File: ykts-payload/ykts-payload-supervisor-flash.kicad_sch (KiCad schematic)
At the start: 10 parts, among them U10 AMS1117-3.3, U11 AT25DF161-SF-T

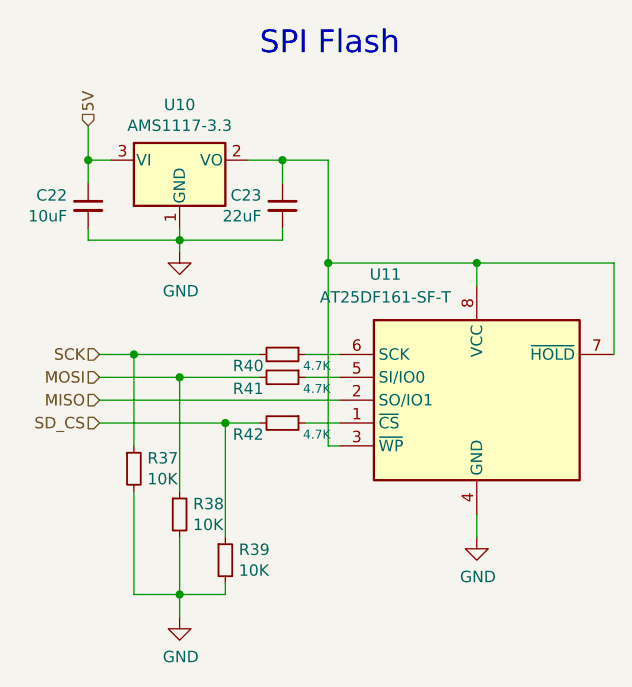
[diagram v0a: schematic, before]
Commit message: Changed flash LDO to L78L33
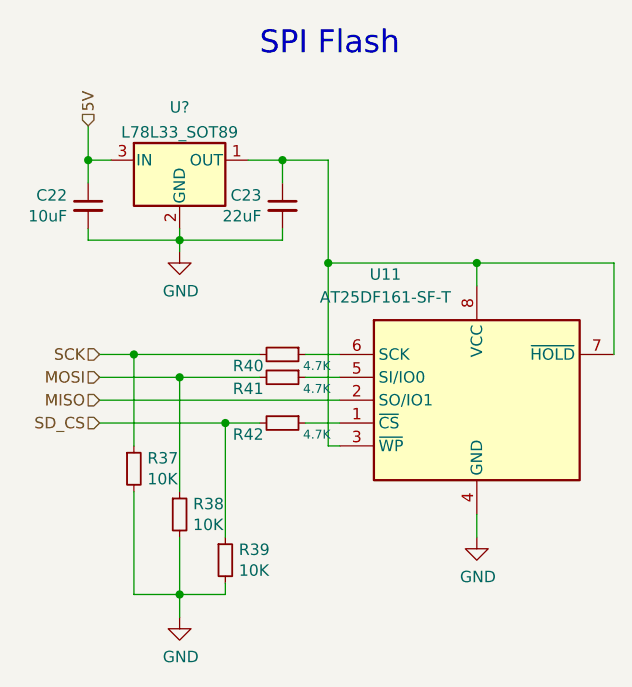
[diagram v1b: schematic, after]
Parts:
- removed U10: AMS1117-3.3, Package_TO_SOT_SMD:SOT-89-3, symbol Regulator_Linear:AMS1117-3.3
- added U?: L78L33_SOT89, Package_TO_SOT_SMD:SOT-89-3, symbol Regulator_Linear:L78L33_SOT89
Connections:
- net 5V: now also U?.3 (IN)
- net GND: now also U?.2 (GND)
- net at C23.1, U11.3 (~{WP}), U11.7 (~{HOLD})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: now also U?.1 (OUT)
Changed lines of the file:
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@@
     (pin "2")
-  )
-  (symbol (lib_id "Regulator_Linear:AMS1117-3.3") (at 132.08 74.93 0)
-    (in_bom yes) (on_board yes)
-    (property "Reference" "U10" (id 0) (at 132.08 68.7832 0))
-    (property "Value" "AMS1117-3.3" (id 1) (at 132.08 71.0946 0))
-    (property "Footprint" "Package_TO_SOT_SMD:SOT-89-3" (id 2) (at 132.08 69.85 0)
-      (effects (font (size 1.27 1.27)) hide)
-    )
-    (property "Datasheet" "http://www.advanced-monolithic.com/pdf/ds1117.pdf" (id 3) (at 134.62 81.28 0)
-      (effects (font (size 1.27 1.27)) hide)
-    )
-    (pin "1")
-    (pin "2")
-    (pin "3")
   )
   (symbol (lib_id "Device:R_Small") (at 127 109.22 0)
@@
     (pin "2")
   )
+  (symbol (lib_id "Regulator_Linear:L78L33_SOT89") (at 132.08 74.93 0)
+    (in_bom yes) (on_board yes) (fields_autoplaced)
+    (property "Reference" "U?" (id 0) (at 132.08 69.0585 0))
+    (property "Value" "L78L33_SOT89" (id 1) (at 132.08 71.8336 0))
+    (property "Footprint" "Package_TO_SOT_SMD:SOT-89-3" (id 2) (at 132.08 69.85 0)
+      (effects (font (size 1.27 1.27) italic) hide)
+    )
+    (property "Datasheet" "http://www.st.com/content/ccc/resource/technical/document/datasheet/15/55/e5/aa/23/5b/43/fd/CD00000446.pdf/files/CD00000446.pdf/jcr:content/translations/en.CD00000446.pdf" (id 3) (at 132.08 76.2 0)
+      (effects (font (size 1.27 1.27)) hide)
+    )
+    (pin "1")
+    (pin "2")
+    (pin "3")
+  )
   (symbol (lib_id "power:GND") (at 165.1 116.84 0)
